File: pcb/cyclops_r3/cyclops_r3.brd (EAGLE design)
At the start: 69.8 x 53.3 mm, 113 parts, among them M12_TUBE_MOUNT PT-LH001, Q1 SUM11006, Q2 IRF540, U1 MCP4921, U10 AD829, U11 MIC5225, U12 MIC5270, U2 317-N, U3 TLV37, U4 337-N, U5 ADR03, U6 OP1177, U7 TLV2374, U8 ZXTD45, U9 ADA4899

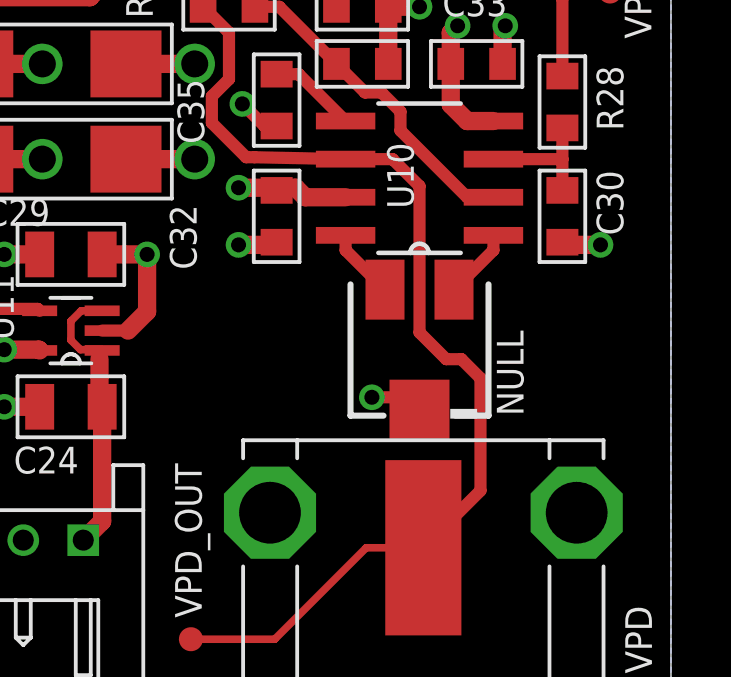
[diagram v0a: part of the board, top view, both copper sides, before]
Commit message: Minor.
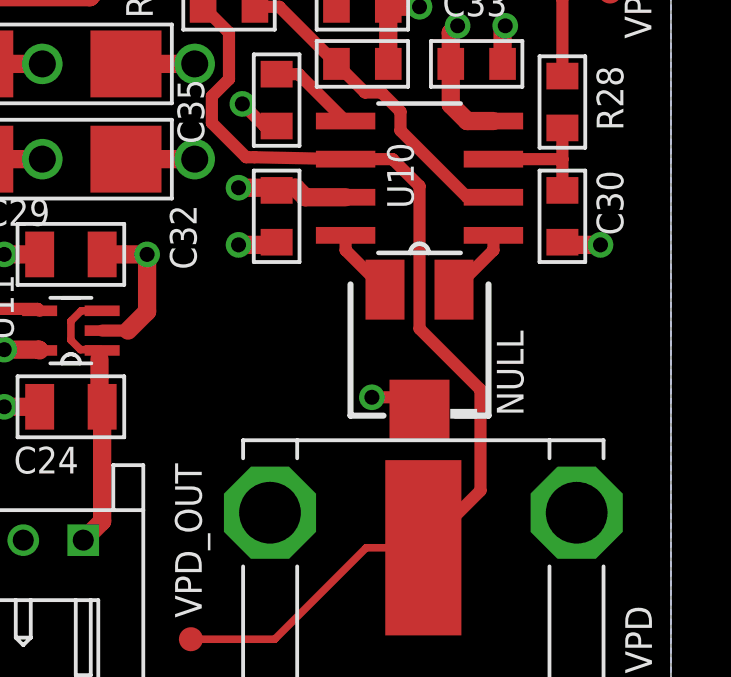
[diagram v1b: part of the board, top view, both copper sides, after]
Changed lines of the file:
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@@
 <layer number="27" name="tValues" color="7" fill="1" visible="yes" active="yes"/>
 <layer number="28" name="bValues" color="7" fill="1" visible="yes" active="yes"/>
-<layer number="29" name="tStop" color="7" fill="3" visible="yes" active="yes"/>
+<layer number="29" name="tStop" color="7" fill="3" visible="no" active="yes"/>
 <layer number="30" name="bStop" color="7" fill="6" visible="no" active="yes"/>
 <layer number="31" name="tCream" color="7" fill="4" visible="no" active="yes"/>
@@
 <contactref element="VPD" pad="1"/>
 <wire x1="90.805" y1="4.826" x2="92.71" y2="6.731" width="0.4064" layer="1"/>
-<wire x1="92.71" y1="6.731" x2="93.726" y2="7.747" width="0" layer="19" extent="1-16"/>
 <wire x1="89.779975" y1="17.78" x2="88.2142" y2="17.78" width="0.4064" layer="1"/>
 <wire x1="85.1789" y1="17.8435" x2="88.2142" y2="17.78" width="0.4064" layer="1"/>
@@
 <wire x1="83.7565" y1="19.8755" x2="84.328" y2="20.447" width="0.4064" layer="1"/>
 <wire x1="89.779975" y1="17.78" x2="90.678" y2="16.881975" width="0.4064" layer="1"/>
-<wire x1="90.678" y1="16.881975" x2="90.678" y2="12.0015" width="0.4064" layer="1"/>
-<wire x1="90.678" y1="12.0015" x2="91.567" y2="11.1125" width="0.4064" layer="1"/>
-<wire x1="91.567" y1="11.1125" x2="92.075" y2="11.1125" width="0.4064" layer="1"/>
-<wire x1="92.075" y1="11.1125" x2="92.71" y2="10.4775" width="0.4064" layer="1"/>
-<wire x1="92.71" y1="10.4775" x2="92.71" y2="6.731" width="0.4064" layer="1"/>
+<wire x1="90.678" y1="16.881975" x2="90.678" y2="12.1285" width="0.4064" layer="1"/>
+<wire x1="92.71" y1="10.0965" x2="92.71" y2="6.731" width="0.4064" layer="1"/>
+<wire x1="90.678" y1="12.1285" x2="92.71" y2="10.0965" width="0.4064" layer="1"/>
 </signal>
 <signal name="N$23">
